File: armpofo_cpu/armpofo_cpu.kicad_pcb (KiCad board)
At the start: 2 copper layers, 185.1 x 74 mm, 86 parts, among them J1 USB_OTG, J2 Conn_01x01, J3 Conn_01x01, J4 Conn_01x16, J5 Conn_01x20, J6 Conn_02x16_Odd_Even, J7 Conn_01x08, J8 Micro_SD_Card, Q1 Q_PMOS_GDS, Q2 Q_PMOS_GDS, Q3 Q_PMOS_GDS, U1 TPS63802, U2 TLV62568DBV, U3 INA181, U4 STM32H750VB, U5 W25Q32JVSS, Y1 25MHz, Y2 32.768 kHz

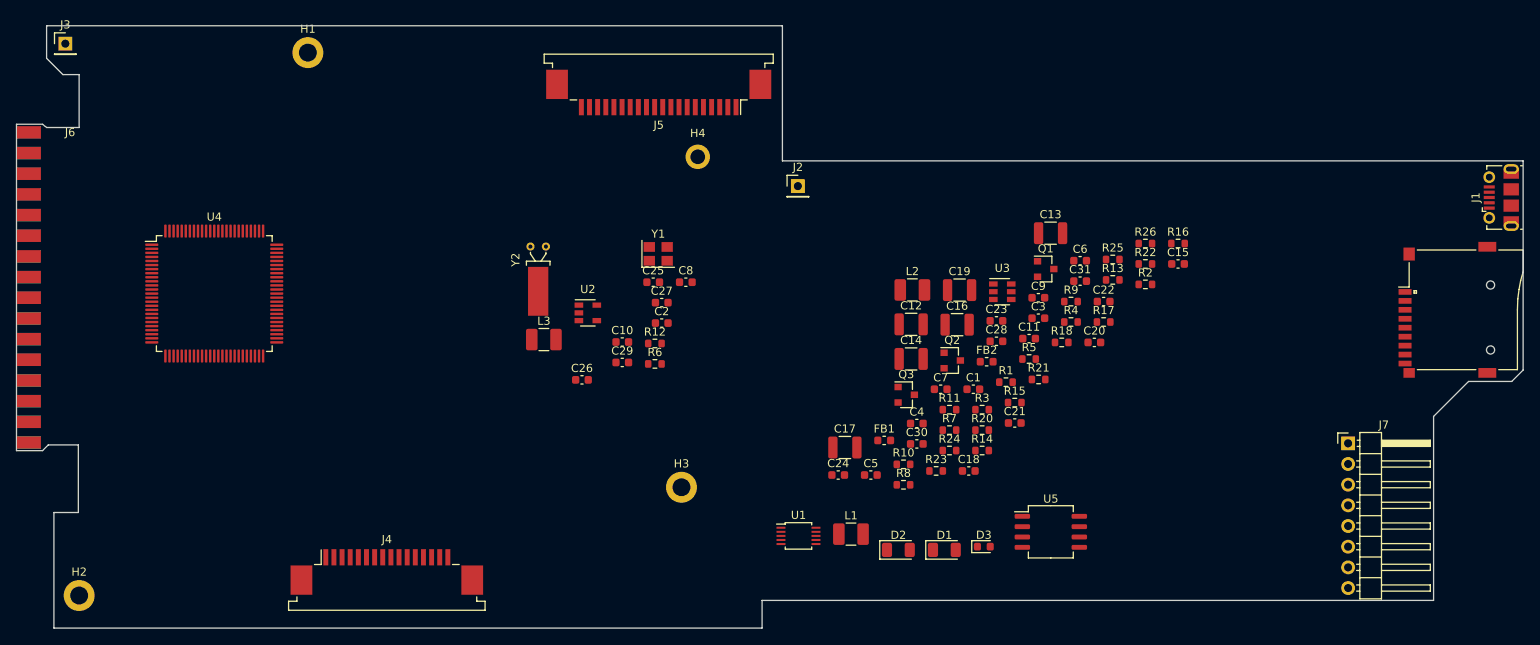
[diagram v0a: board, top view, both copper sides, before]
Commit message: some progress
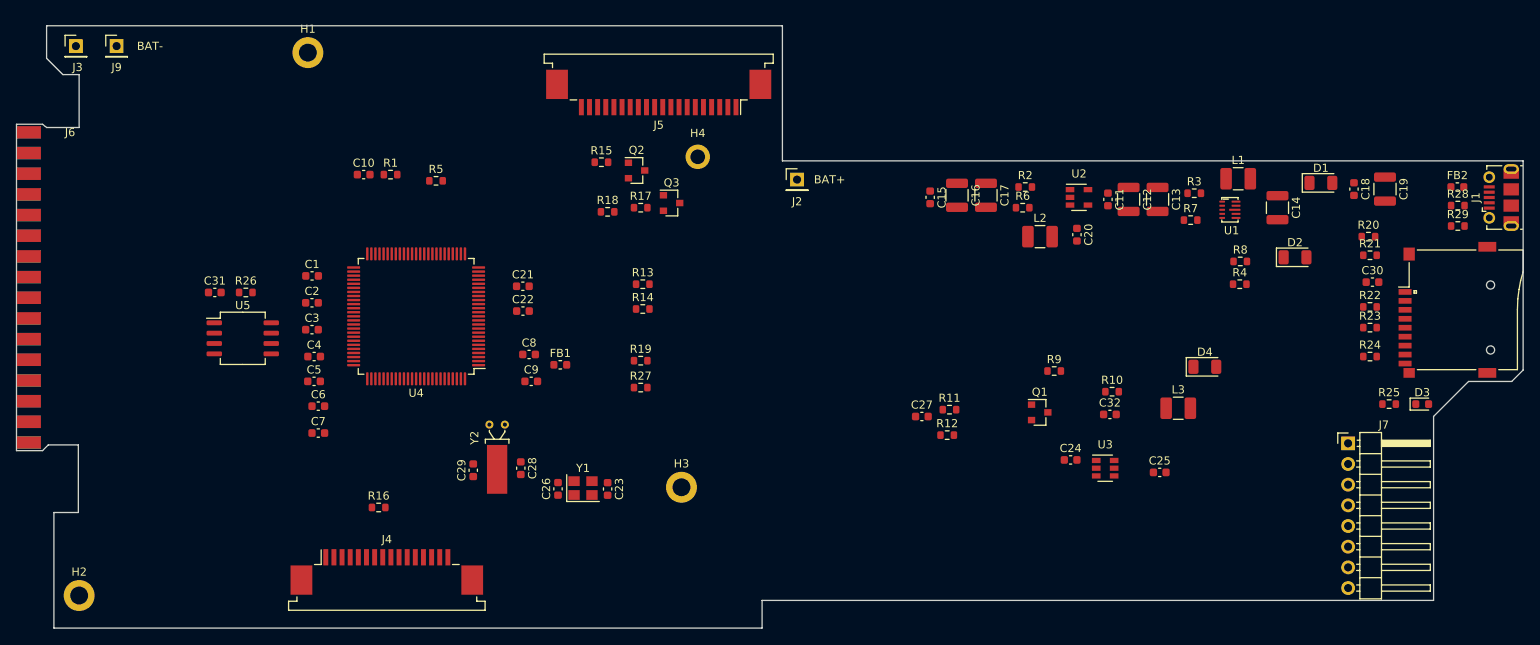
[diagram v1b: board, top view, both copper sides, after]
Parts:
- added C32: 1nF, Capacitor_SMD:C_0603_1608Metric, F.Cu at (202.7, 117.8)
- added D4: SS24, Diode_SMD:D_1206_3216Metric, F.Cu at (214.4, 111.9)
- added J9: Conn_01x01, Connector_PinHeader_2.54mm:PinHeader_1x01_P2.54mm_Vertical, F.Cu at (80.7, 72.5)
- added R19: 100k, Resistor_SMD:R_0603_1608Metric, F.Cu at (145.1, 111.1)
- added R27: 100k, Resistor_SMD:R_0603_1608Metric, F.Cu at (145.1, 114.5)
- added R28: 22R, Resistor_SMD:R_0603_1608Metric, F.Cu at (245.5, 92.1)
- added R29: 22R, Resistor_SMD:R_0603_1608Metric, F.Cu at (245.5, 94.6)
- U1: footprint Package_SO:TSSOP-10_3x3mm_P0.5mm -> PROJECT_LOCAL:DLA0010A
- moved R26 110.7 mm to (96.6, 102.8)
- moved C31 106.3 mm to (92.8, 102.8)
- moved R16 103.4 mm to (112.9, 129.2)
- moved U5 102.1 mm to (96.2, 108.4)
- moved C6 95.3 mm to (105.5, 116.7)
- moved C3 89.3 mm to (104.7, 107.3)
- moved C1 82.4 mm to (104.7, 100.7)
- moved R1 79.8 mm to (114.4, 88.3)
- moved L3 78.4 mm to (211.1, 117.0)
- moved C7 76.7 mm to (105.5, 120.0)
- moved R5 76.1 mm to (119.9, 89.0)
- moved C4 74.5 mm to (105.0, 110.6)
- moved C22 71.3 mm to (130.6, 105.1)
- moved C5 69.4 mm to (105.0, 113.7)
- moved C25 66.5 mm to (208.9, 124.9)
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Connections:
- net /5V-INPUT renamed /3-5V
- J1 pad 2: /USB-DM -> Net-(J1-Pad2)
- J1 pad 3: /USB-DP -> Net-(J1-Pad3)
- U4 pad 15: /LED1 -> /ADC-5V
- U4 pad 62: Net-(U4-Pad62) -> /LED1
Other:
- board text added: "BAT+"
- board text added: "BAT-"
